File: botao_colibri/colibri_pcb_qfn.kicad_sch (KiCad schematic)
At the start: 6 parts, among them J2 TC2030, U1 ME54BS12

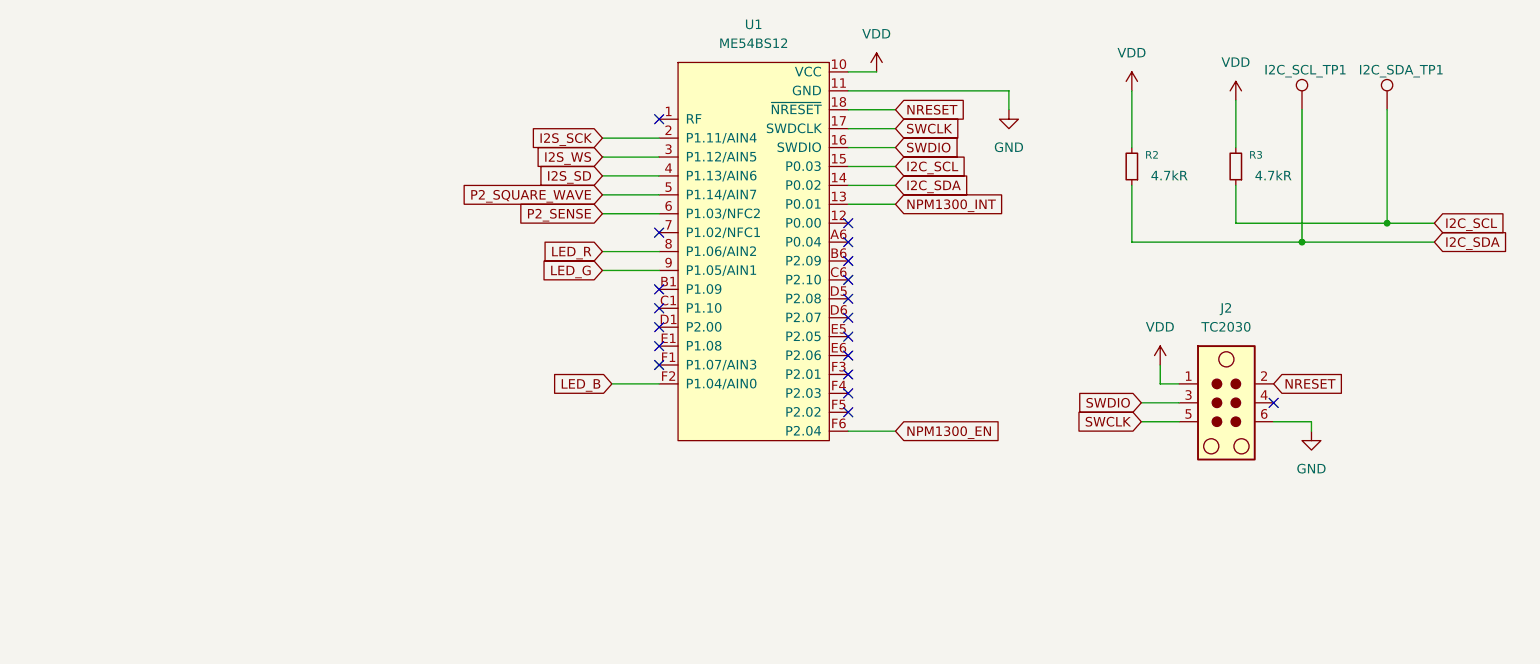
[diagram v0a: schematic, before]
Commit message: Desenho dos pads do botão principal, GPIOS acessíveis (adição de conectores para as GPIOS sem uso atual), retrabalho de trilhas.
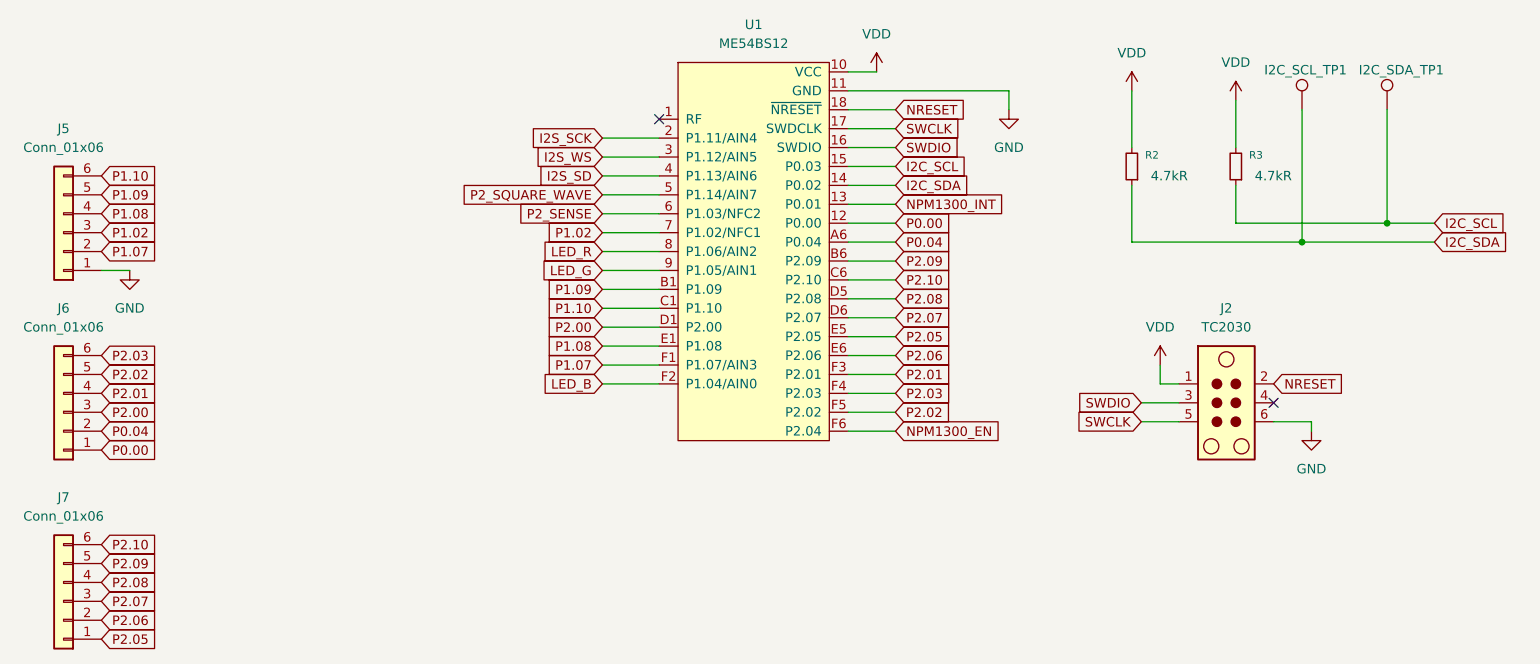
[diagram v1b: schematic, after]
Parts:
- added J5, J6, J7: Conn_01x06, Connector_PinHeader_2.54mm:PinHeader_1x06_P2.54mm_Vertical, symbol Connector_Generic:Conn_01x06
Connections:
- net GND: now also J5.1 (Pin_1)
- net P0.00: now reaches U1.12 (P0.00)
- net P0.00: now also J6.1 (Pin_1)
- net P1.02: now reaches U1.7 (P1.02/NFC1)
- net P1.02: now also J5.3 (Pin_3)
- net P0.04: now reaches U1.A6 (P0.04)
- net P0.04: now also J6.2 (Pin_2)
- net P1.09: now reaches U1.B1 (P1.09)
- net P1.09: now also J5.5 (Pin_5)
- net P2.09: now reaches U1.B6 (P2.09)
- net P2.09: now also J7.5 (Pin_5)
- net P1.10: now reaches U1.C1 (P1.10)
- net P1.10: now also J5.6 (Pin_6)
- net P2.10: now reaches U1.C6 (P2.10)
- net P2.10: now also J7.6 (Pin_6)
- net P2.00: now reaches U1.D1 (P2.00)
- net P2.00: now also J6.3 (Pin_3)
- net P2.08: now reaches U1.D5 (P2.08)
- net P2.08: now also J7.4 (Pin_4)
- net P2.07: now reaches U1.D6 (P2.07)
- net P2.07: now also J7.3 (Pin_3)
- net P1.08: now reaches U1.E1 (P1.08)
- net P1.08: now also J5.4 (Pin_4)
- net P2.05: now reaches U1.E5 (P2.05)
- net P2.05: now also J7.1 (Pin_1)
- net P2.06: now reaches U1.E6 (P2.06)
- net P2.06: now also J7.2 (Pin_2)
- net P1.07: now reaches U1.F1 (P1.07/AIN3)
- net P1.07: now also J5.2 (Pin_2)
- net P2.01: now reaches U1.F3 (P2.01)
- net P2.01: now also J6.4 (Pin_4)
- net P2.03: now reaches U1.F4 (P2.03)
- net P2.03: now also J6.6 (Pin_6)
- net P2.02: now reaches U1.F5 (P2.02)
- net P2.02: now also J6.5 (Pin_5)
- no-connect marks 19 -> 2

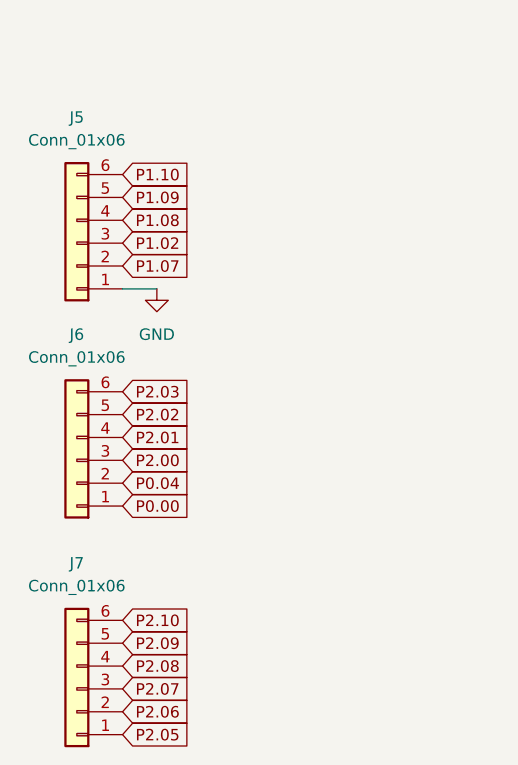
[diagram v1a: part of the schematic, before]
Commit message: continuação
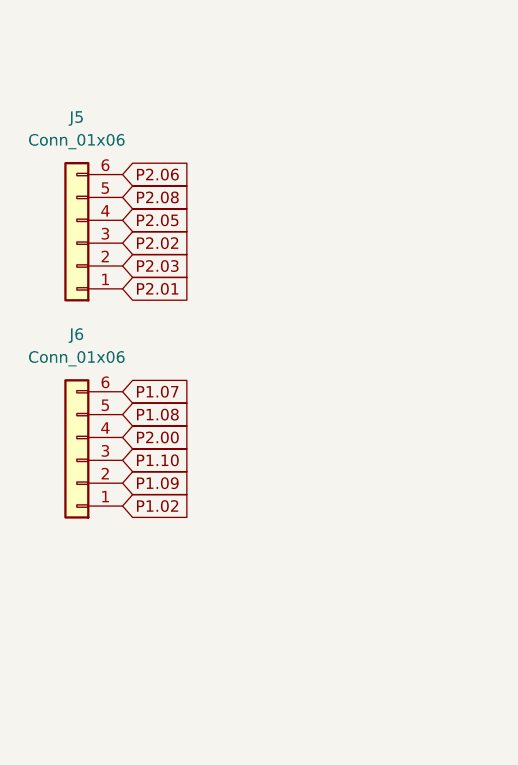
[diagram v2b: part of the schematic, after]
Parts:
- removed J7: Conn_01x06, Connector_PinHeader_2.54mm:PinHeader_1x06_P2.54mm_Vertical, symbol Connector_Generic:Conn_01x06
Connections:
- net GND: no longer J5.1 (Pin_1)
- net P0.00: no longer J6.1 (Pin_1)
- net P0.04: no longer J6.2 (Pin_2)
- net P1.02: now also J6.1 (Pin_1); no longer J5.3 (Pin_3)
- net P1.07: now also J6.6 (Pin_6); no longer J5.2 (Pin_2)
- net P1.08: now also J6.5 (Pin_5); no longer J5.4 (Pin_4)
- net P1.09: now also J6.2 (Pin_2); no longer J5.5 (Pin_5)
- net P1.10: now also J6.3 (Pin_3); no longer J5.6 (Pin_6)
- net P2.00: now also J6.4 (Pin_4); no longer J6.3 (Pin_3)
- net P2.01: now also J5.1 (Pin_1); no longer J6.4 (Pin_4)
- net P2.02: now also J5.3 (Pin_3); no longer J6.5 (Pin_5)
- net P2.03: now also J5.2 (Pin_2); no longer J6.6 (Pin_6)
- net P2.05: now also J5.4 (Pin_4)
- net P2.06: now also J5.6 (Pin_6)
- net P2.08: now also J5.5 (Pin_5)
